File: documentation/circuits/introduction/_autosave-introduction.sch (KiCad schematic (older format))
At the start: 16 parts

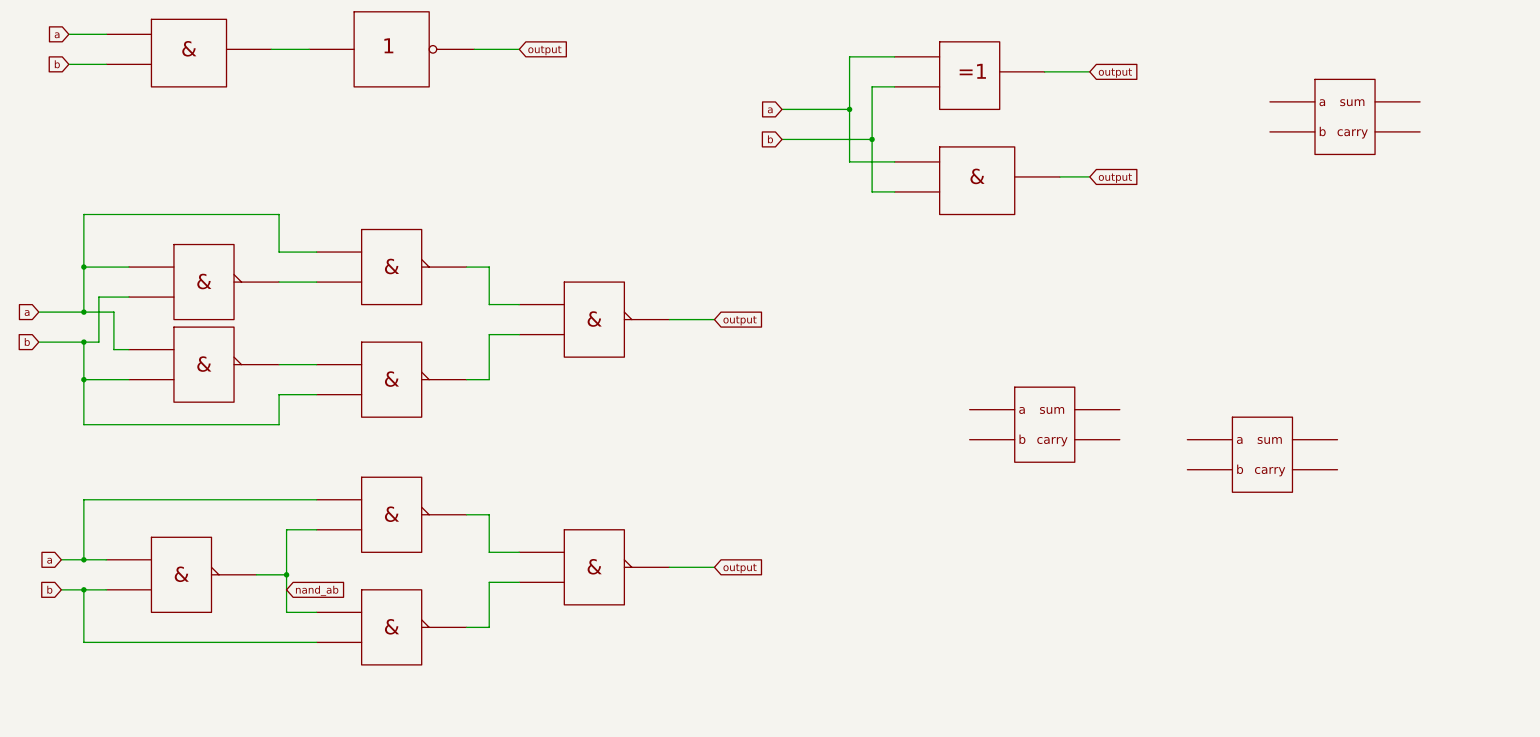
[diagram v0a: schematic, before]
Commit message: update
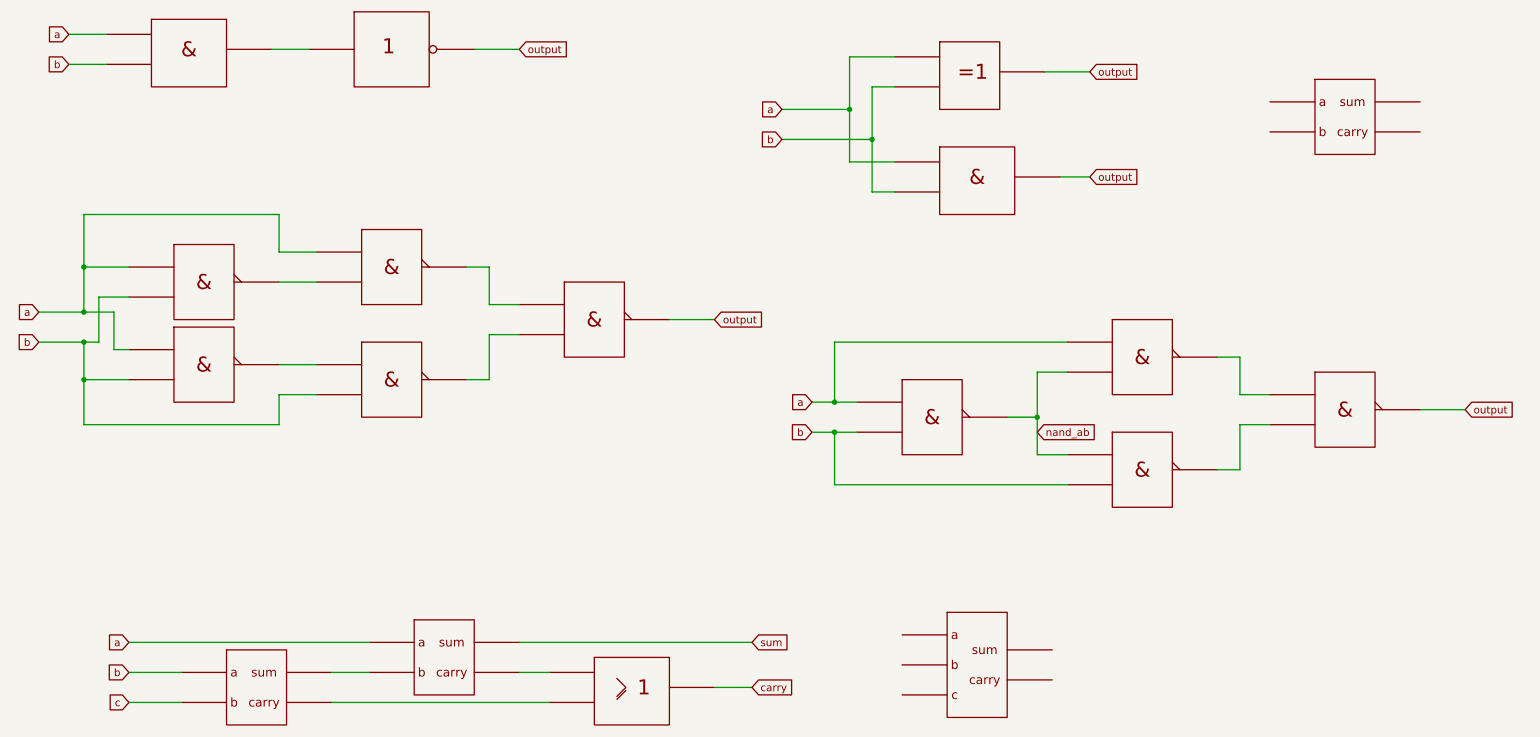
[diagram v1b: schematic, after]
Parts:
- added U?: 7432, symbol disimpy:7432
- added U?: full_adder, symbol disimpy:full_adder
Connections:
- net a: now also U?.~
- net b: now also U?.~
- net c: now reaches U?.~
- net sum: now reaches U?.~
- new net: U?.~, U?.~ (x10)
- new net carry: U?.~
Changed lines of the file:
@@
 L introduction-rescue:7400-dismpy U?
 U 1 1 5E33AC9E
-P 3150 4250
-F 0 "U?" H 3400 4550 50  0001 C CNN
-F 1 "7400" H 3350 3950 50  0001 C CNN
-F 2 "" H 3150 4250 50  0001 C CNN
-F 3 "" H 3150 4250 50  0001 C CNN
-	1    3150 4250
+P 8150 3200
+F 0 "U?" H 8400 3500 50  0001 C CNN
+F 1 "7400" H 8350 2900 50  0001 C CNN
+F 2 "" H 8150 3200 50  0001 C CNN
+F 3 "" H 8150 3200 50  0001 C CNN
+	1    8150 3200
 	1    0    0    -1
 $EndComp
@@
 L introduction-rescue:7400-dismpy U?
 U 1 1 5E33BC4E
-P 1750 4650
-F 0 "U?" H 2000 4950 50  0001 C CNN
-F 1 "7400" H 1950 4350 50  0001 C CNN
-F 2 "" H 1750 4650 50  0001 C CNN
-F 3 "" H 1750 4650 50  0001 C CNN
-	1    1750 4650
+P 6750 3600
+F 0 "U?" H 7000 3900 50  0001 C CNN
+F 1 "7400" H 6950 3300 50  0001 C CNN
+F 2 "" H 6750 3600 50  0001 C CNN
+F 3 "" H 6750 3600 50  0001 C CNN
+	1    6750 3600
 	1    0    0    -1
 $EndComp
@@
 L introduction-rescue:7400-dismpy U?
 U 1 1 5E33D300
-P 3150 5000
-F 0 "U?" H 3400 5300 50  0001 C CNN
-F 1 "7400" H 3350 4700 50  0001 C CNN
-F 2 "" H 3150 5000 50  0001 C CNN
-F 3 "" H 3150 5000 50  0001 C CNN
-	1    3150 5000
+P 8150 3950
+F 0 "U?" H 8400 4250 50  0001 C CNN
+F 1 "7400" H 8350 3650 50  0001 C CNN
+F 2 "" H 8150 3950 50  0001 C CNN
+F 3 "" H 8150 3950 50  0001 C CNN
+	1    8150 3950
 	1    0    0    -1
 $EndComp
@@
 L introduction-rescue:7400-dismpy U?
 U 1 1 5E33DBBB
-P 4500 4600
-F 0 "U?" H 4750 4900 50  0001 C CNN
-F 1 "7400" H 4700 4300 50  0001 C CNN
-F 2 "" H 4500 4600 50  0001 C CNN
-F 3 "" H 4500 4600 50  0001 C CNN
-	1    4500 4600
-	1    0    0    -1
-$EndComp
-Text GLabel 950  4550 0    50   Input ~ 0
+P 9500 3550
+F 0 "U?" H 9750 3850 50  0001 C CNN
+F 1 "7400" H 9700 3250 50  0001 C CNN
+F 2 "" H 9500 3550 50  0001 C CNN
+F 3 "" H 9500 3550 50  0001 C CNN
+	1    9500 3550
+	1    0    0    -1
+$EndComp
+Text GLabel 5950 3500 0    50   Input ~ 0
 a
-Text GLabel 950  4750 0    50   Input ~ 0
+Text GLabel 5950 3700 0    50   Input ~ 0
 b
-Text GLabel 5300 4600 2    50   Input ~ 0
-output
-Wire Wire Line
-	2650 4350 2450 4350
-Wire Wire Line
-	2450 4350 2450 4650
-Wire Wire Line
-	2450 4900 2650 4900
-Wire Wire Line
-	2250 4650 2450 4650
-Connection ~ 2450 4650
-Wire Wire Line
-	2450 4650 2450 4900
-Wire Wire Line
-	950  4550 1100 4550
-Wire Wire Line
-	2650 4150 1100 4150
-Wire Wire Line
-	1100 4150 1100 4550
-Connection ~ 1100 4550
-Wire Wire Line
-	1100 4550 1250 4550
-Wire Wire Line
-	3650 4250 3800 4250
-Wire Wire Line
-	3800 4250 3800 4500
-Wire Wire Line
-	3800 4500 4000 4500
-Wire Wire Line
-	4000 4700 3800 4700
-Wire Wire Line
-	3800 4700 3800 5000
-Wire Wire Line
-	3800 5000 3650 5000
-Wire Wire Line
-	5300 4600 5000 4600
-Wire Wire Line
-	950  4750 1100 4750
-Connection ~ 1100 4750
-Wire Wire Line
-	1100 4750 1250 4750
-Wire Wire Line
-	1100 5100 2650 5100
-Wire Wire Line
-	1100 4750 1100 5100
+Text GLabel 10300 3550 2    50   Input ~ 0
+output
+Wire Wire Line
+	7650 3300 7450 3300
+Wire Wire Line
+	7450 3300 7450 3600
+Wire Wire Line
+	7450 3850 7650 3850
+Wire Wire Line
+	7250 3600 7450 3600
+Connection ~ 7450 3600
+Wire Wire Line
+	7450 3600 7450 3850
+Wire Wire Line
+	5950 3500 6100 3500
+Wire Wire Line
+	7650 3100 6100 3100
+Wire Wire Line
+	6100 3100 6100 3500
+Connection ~ 6100 3500
+Wire Wire Line
+	6100 3500 6250 3500
+Wire Wire Line
+	8650 3200 8800 3200
+Wire Wire Line
+	8800 3200 8800 3450
+Wire Wire Line
+	8800 3450 9000 3450
+Wire Wire Line
+	9000 3650 8800 3650
+Wire Wire Line
+	8800 3650 8800 3950
+Wire Wire Line
+	8800 3950 8650 3950
+Wire Wire Line
+	10300 3550 10000 3550
+Wire Wire Line
+	5950 3700 6100 3700
+Connection ~ 6100 3700
+Wire Wire Line
+	6100 3700 6250 3700
+Wire Wire Line
+	6100 4050 7650 4050
+Wire Wire Line
+	6100 3700 6100 4050
 $Comp
 L introduction-rescue:7400-dismpy U?
@@
 Wire Wire Line
 	800  2900 1100 2900
-Text GLabel 2450 4750 2    50   Input ~ 0
+Text GLabel 7450 3700 2    50   Input ~ 0
 nand_ab
 $Comp
@@
 L disimpy:half_adder U?
 U 1 1 5E3465F5
-P 7500 3650
-F 0 "U?" H 7750 3950 50  0001 C CNN
-F 1 "half_adder" H 7700 3350 50  0001 C CNN
-F 2 "" H 7500 3650 50  0001 C CNN
-F 3 "" H 7500 3650 50  0001 C CNN
-	1    7500 3650
+P 2250 5400
+F 0 "U?" H 2500 5700 50  0001 C CNN
+F 1 "half_adder" H 2450 5100 50  0001 C CNN
+F 2 "" H 2250 5400 50  0001 C CNN
+F 3 "" H 2250 5400 50  0001 C CNN
+	1    2250 5400
 	1    0    0    -1
 $EndComp
@@
 L disimpy:half_adder U?
 U 1 1 5E346EA0
-P 8950 3850
-F 0 "U?" H 9200 4150 50  0001 C CNN
-F 1 "half_adder" H 9150 3550 50  0001 C CNN
-F 2 "" H 8950 3850 50  0001 C CNN
-F 3 "" H 8950 3850 50  0001 C CNN
-	1    8950 3850
-	1    0    0    -1
-$EndComp
+P 3500 5200
+F 0 "U?" H 3750 5500 50  0001 C CNN
+F 1 "half_adder" H 3700 4900 50  0001 C CNN
+F 2 "" H 3500 5200 50  0001 C CNN
+F 3 "" H 3500 5200 50  0001 C CNN
+	1    3500 5200
+	1    0    0    -1
+$EndComp
+Text GLabel 1400 5100 0    50   Input ~ 0
+a
+Text GLabel 1400 5300 0    50   Input ~ 0
+b
+Text GLabel 1400 5500 0    50   Input ~ 0
+c
+Text GLabel 5550 5100 2    50   Input ~ 0
+sum
+Wire Wire Line
+	3000 5100 1400 5100
+Wire Wire Line
+	1750 5300 1400 5300
+Wire Wire Line
+	1750 5500 1400 5500
+Wire Wire Line
+	3000 5300 2750 5300
+$Comp
+L disimpy:7432 U?
+U 1 1 5E33EB25
+P 4750 5400
+F 0 "U?" H 4850 5650 50  0001 C CNN
+F 1 "7432" H 4900 5100 50  0001 C CNN
+F 2 "" H 4750 5400 50  0001 C CNN
+F 3 "" H 4750 5400 50  0001 C CNN
+	1    4750 5400
+	1    0    0    -1
+$EndComp
+Wire Wire Line
+	4200 5300 4000 5300
+Wire Wire Line
+	2750 5500 4200 5500
+Wire Wire Line
+	4000 5100 5550 5100
+Text GLabel 5550 5400 2    50   Input ~ 0
+carry
+Wire Wire Line
+	5300 5400 5550 5400
+$Comp
+L disimpy:full_adder U?
+U 1 1 5E359015
+P 7050 5150
+F 0 "U?" H 7300 5450 50  0001 C CNN
+F 1 "full_adder" H 7250 4850 50  0001 C CNN
+F 2 "" H 7050 5050 50  0001 C CNN
+F 3 "" H 7050 5050 50  0001 C CNN
+	1    7050 5150
+	1    0    0    -1
+$EndComp
